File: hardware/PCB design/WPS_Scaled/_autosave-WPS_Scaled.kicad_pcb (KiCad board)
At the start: 4 copper layers, 120 x 115 mm, 124 parts, among them J1 KF128-5.08-2P, J10 KF350-3.5-3P, J11 KF350-3.5-3P, J12-A1 KF350-3.5-2P, J12-B1 KF350-3.5-2P, J12-C1 KF350-3.5-2P, J13 ZX-XH2.54-2PZZ, J14 2.54-1*4P母, J15 ZX-XH2.54-2PZZ, J16 ZX-XH2.54-2PZZ, J2 KF128-5.08-2P, J3 KF128-5.08-2P, J4 KF128-5.08-2P, J5 KF350-3.5-3P, J6 KF350-3.5-3P, J7 KF350-3.5-3P, J8-A1 KF350-3.5-2P, J8-B1 KF350-3.5-2P, J9-A1 KF350-3.5-2P, J9-B1 KF350-3.5-2P, K1 SRD-05VDC-SL-C, K2 SRD-05VDC-SL-C, K3 SRD-05VDC-SL-C, Q1 2N2222, Q2 IRF9540NPBF, Q3 2N2222, Q4 2N2222, Q5 2N2222, U1 LM2595T-5.0, U2 TLV1117LV33DCYR, U3 ESP32-S3-WROOM-1(N16R8), U4 TYPEC-306DDW-ARP16, U5 CH340C

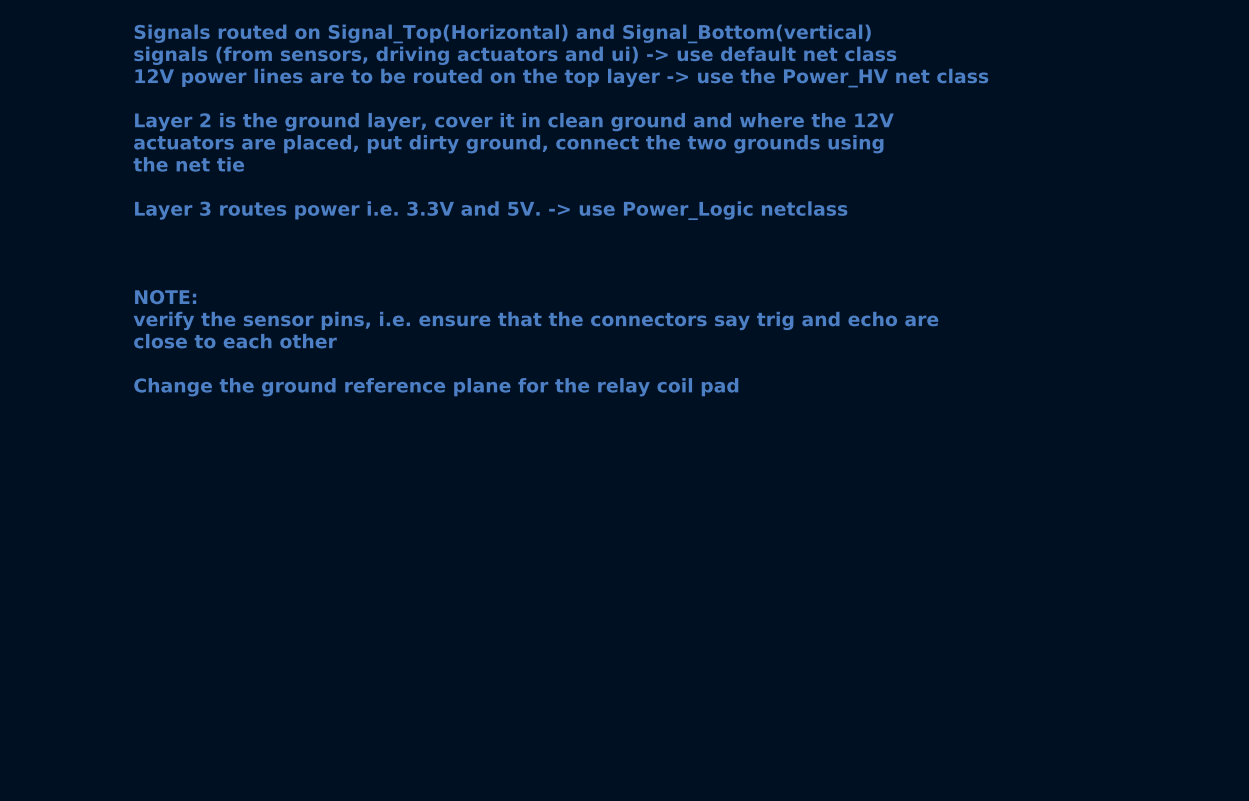
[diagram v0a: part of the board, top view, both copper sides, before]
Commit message: finalized the routing
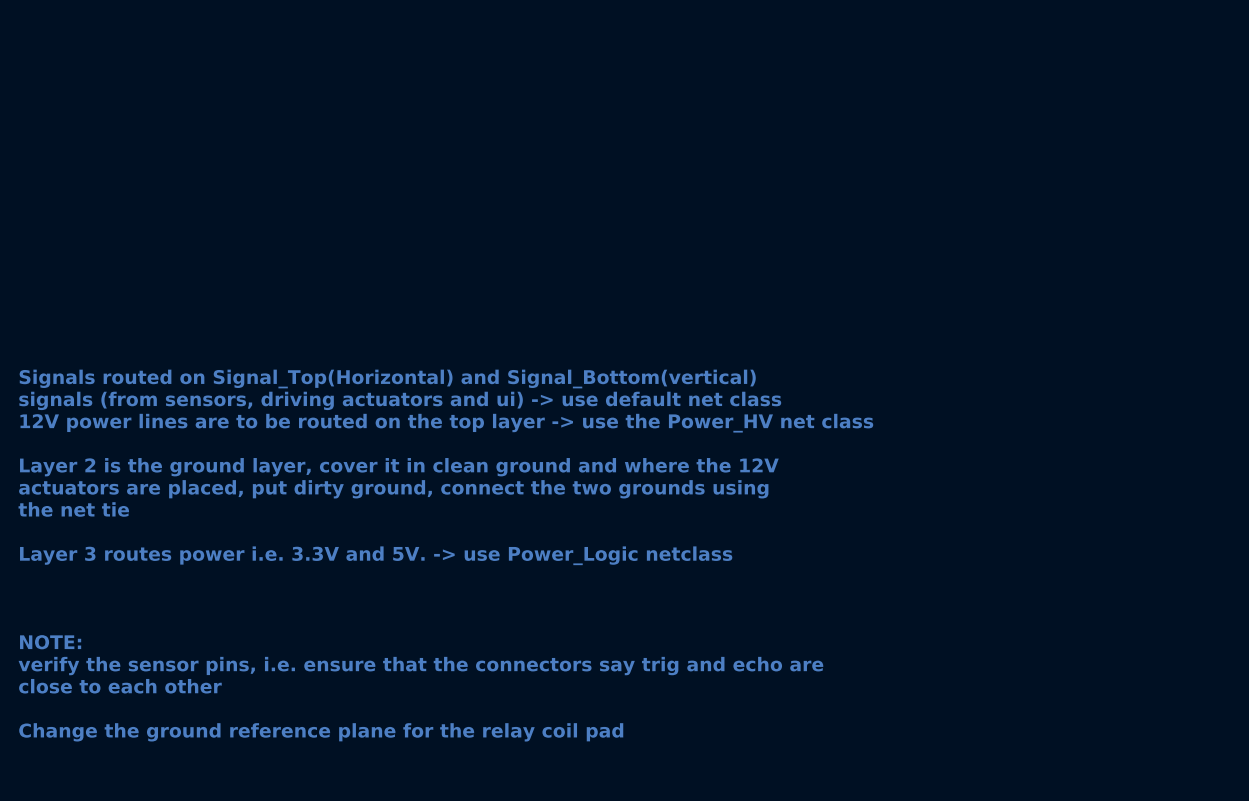
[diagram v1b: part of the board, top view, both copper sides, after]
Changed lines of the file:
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@@
 	)
 	(gr_text "Signals routed on Signal_Top(Horizontal) and Signal_Bottom(vertical)\nsignals (from sensors, driving actuators and ui) -> use default net class\n12V power lines are to be routed on the top layer -> use the Power_HV net class\n\nLayer 2 is the ground layer, cover it in clean ground and where the 12V\nactuators are placed, put dirty ground, connect the two grounds using \nthe net tie\n\nLayer 3 routes power i.e. 3.3V and 5V. -> use Power_Logic netclass\n\n\n\nNOTE:\nverify the sensor pins, i.e. ensure that the connectors say trig and echo are\nclose to each other\n\nChange the ground reference plane for the relay coil pad\n\n"
-		(at -91.44 73.66 0)
+		(at -104.013 111.379 0)
 		(layer "B.Cu")
 		(effects
